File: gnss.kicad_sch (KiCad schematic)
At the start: 26 parts, among them J401 GNSS ANT pads, U401 AT6558R-5N32, X401 TCXO 26MHz, X402 32.768kHz

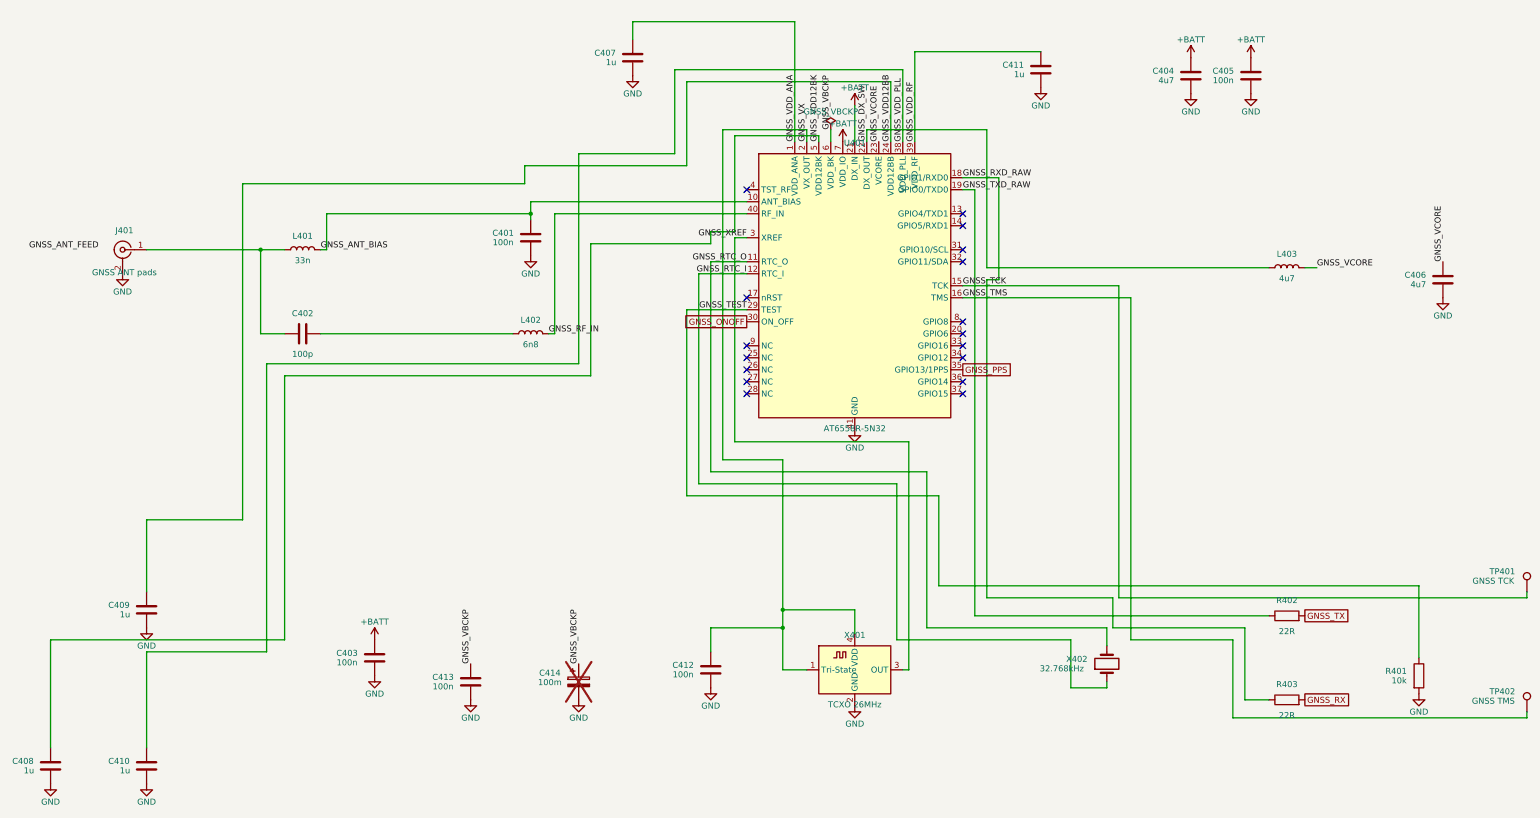
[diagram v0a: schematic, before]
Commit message: Adjust layout and schematic
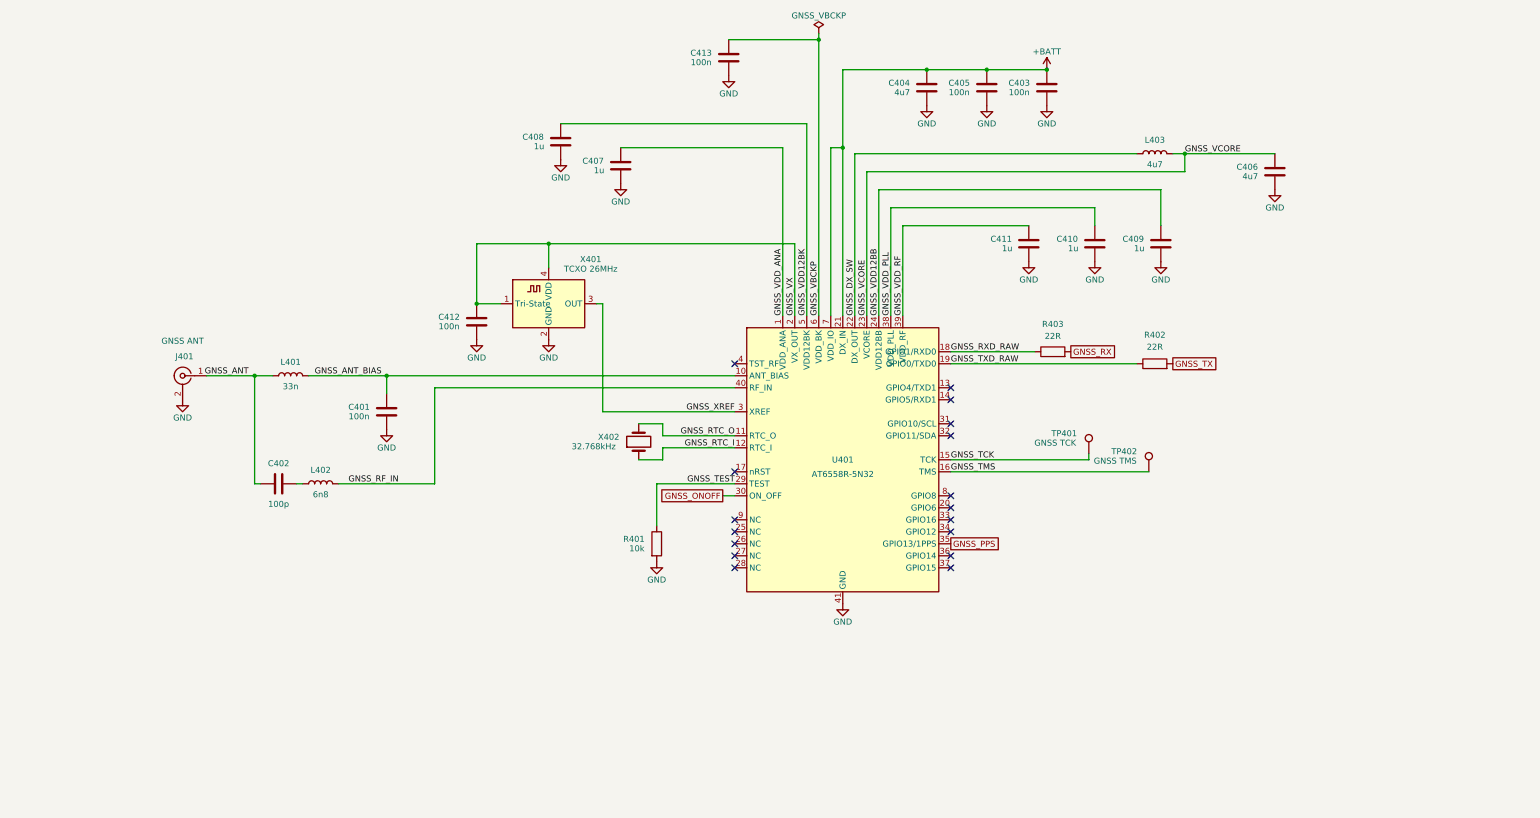
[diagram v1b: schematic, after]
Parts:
- removed C414: 100m, cc1200_balloon:SuperCap_KEMET_FCS_D10.7mm, symbol Device:C_Polarized
- J401: value GNSS ANT pads -> GNSS ANT
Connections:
- net GNSS_ANT: now reaches C402.1, J401.1 (In), L401.1
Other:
- moved on the sheet: C401, C402, C403, C404, C405, C406, C407, C408, C409, C410, C411, C412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
